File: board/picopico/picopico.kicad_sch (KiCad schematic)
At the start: 52 parts, among them J2 display, J3 USB_B_Micro, Q1 BC817, Q2 BC817, SW1 SW_SPDT, SW3 SW_Push, SW5 SW_Push, SW6 SW_Push, SW7 SW_Push, SW8 SW_Push, U1 ESP32-WROVER-E, U2 volume_wheel, U3 AMS1117-3.3, U4 audio, U5 STC4054GR, U6 CH340C

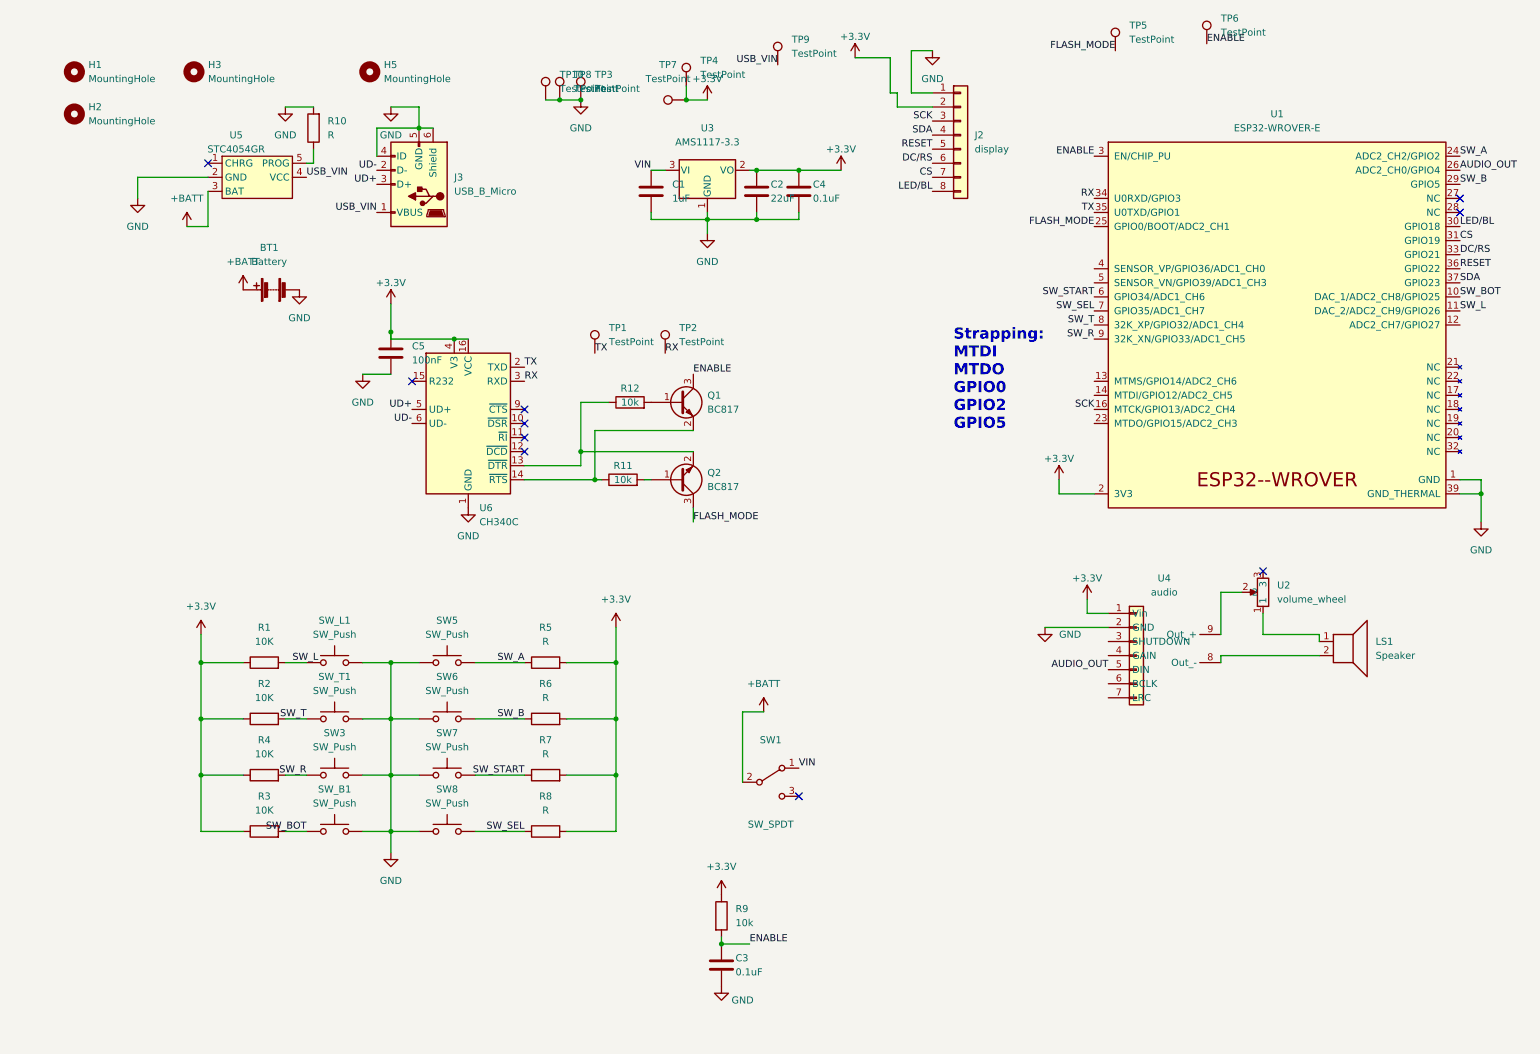
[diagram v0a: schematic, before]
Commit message: more board changes
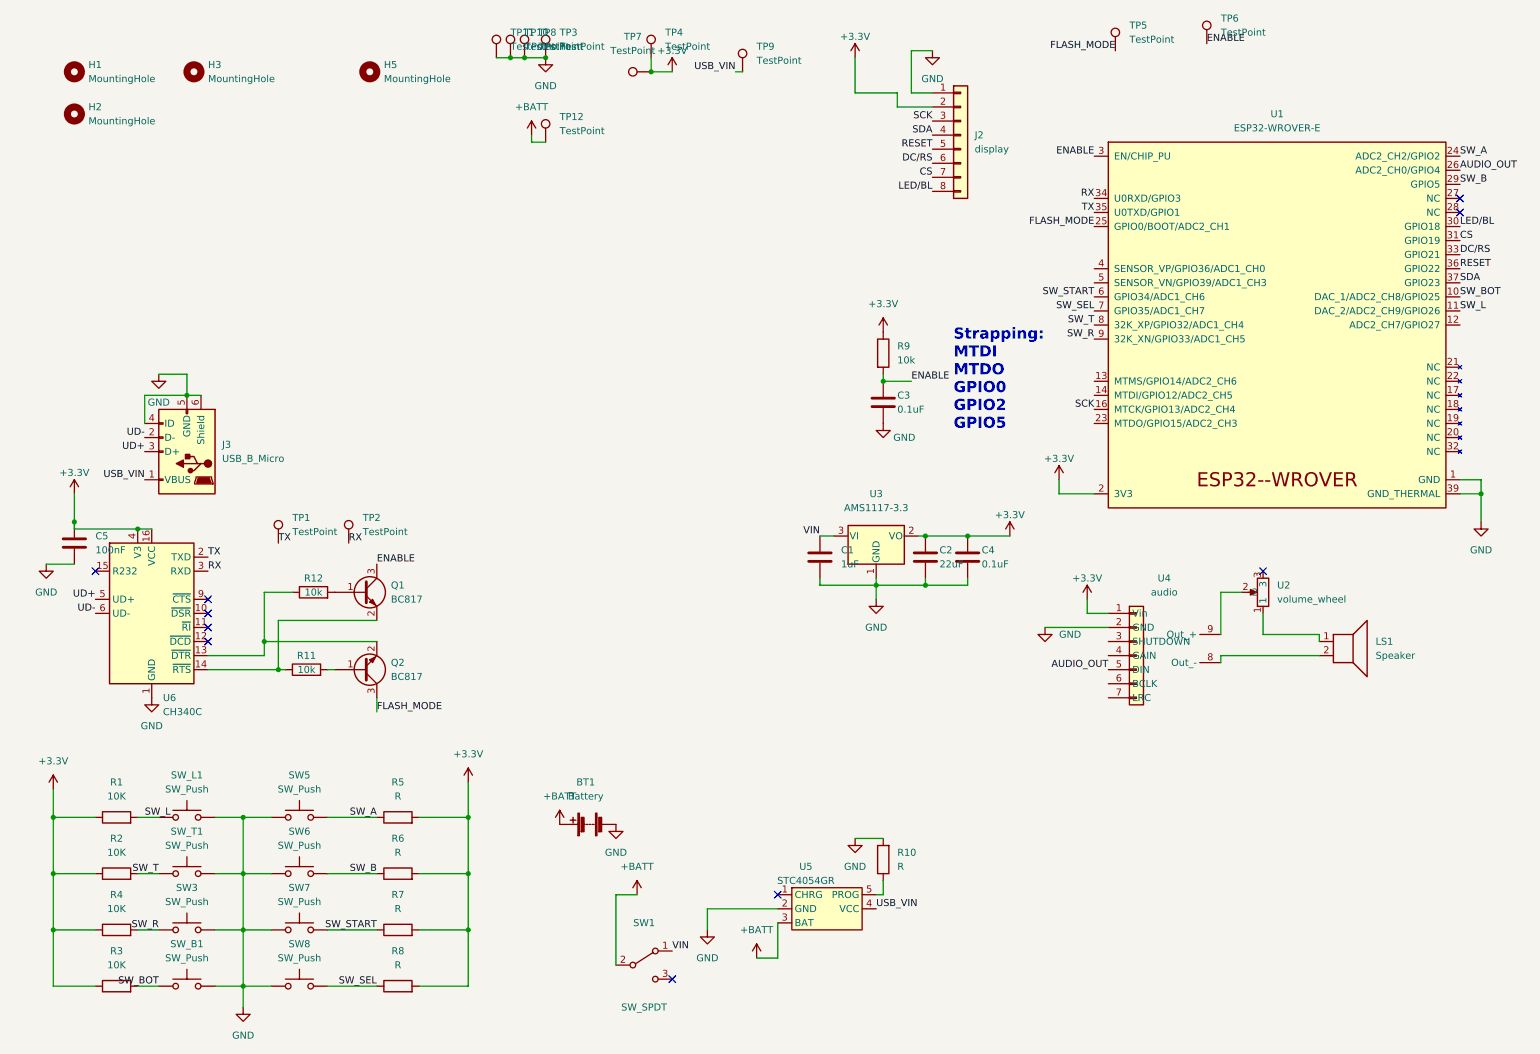
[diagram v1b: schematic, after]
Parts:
- added TP11, TP12: TestPoint, picopico:pad, symbol Connector:TestPoint
- BT1: footprint Connector_JST:JST_PH_S2B-PH-K_1x02_P2.00mm_Horizontal -> picopico:SM02B-SRSS-TB
- SW7, SW8: footprint Button_Switch_SMD:SW_SPST_B3U-1000P -> Button_Switch_SMD:SW_SPST_B3U-1100P-B
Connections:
- net +BATT: now also TP12.1
- net GND: now also TP11.1
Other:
- moved on the sheet: BT1, C1, C2, C3, C4, C5, J3, Q1, Q2, R1, R10, R11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

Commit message: more board stuff
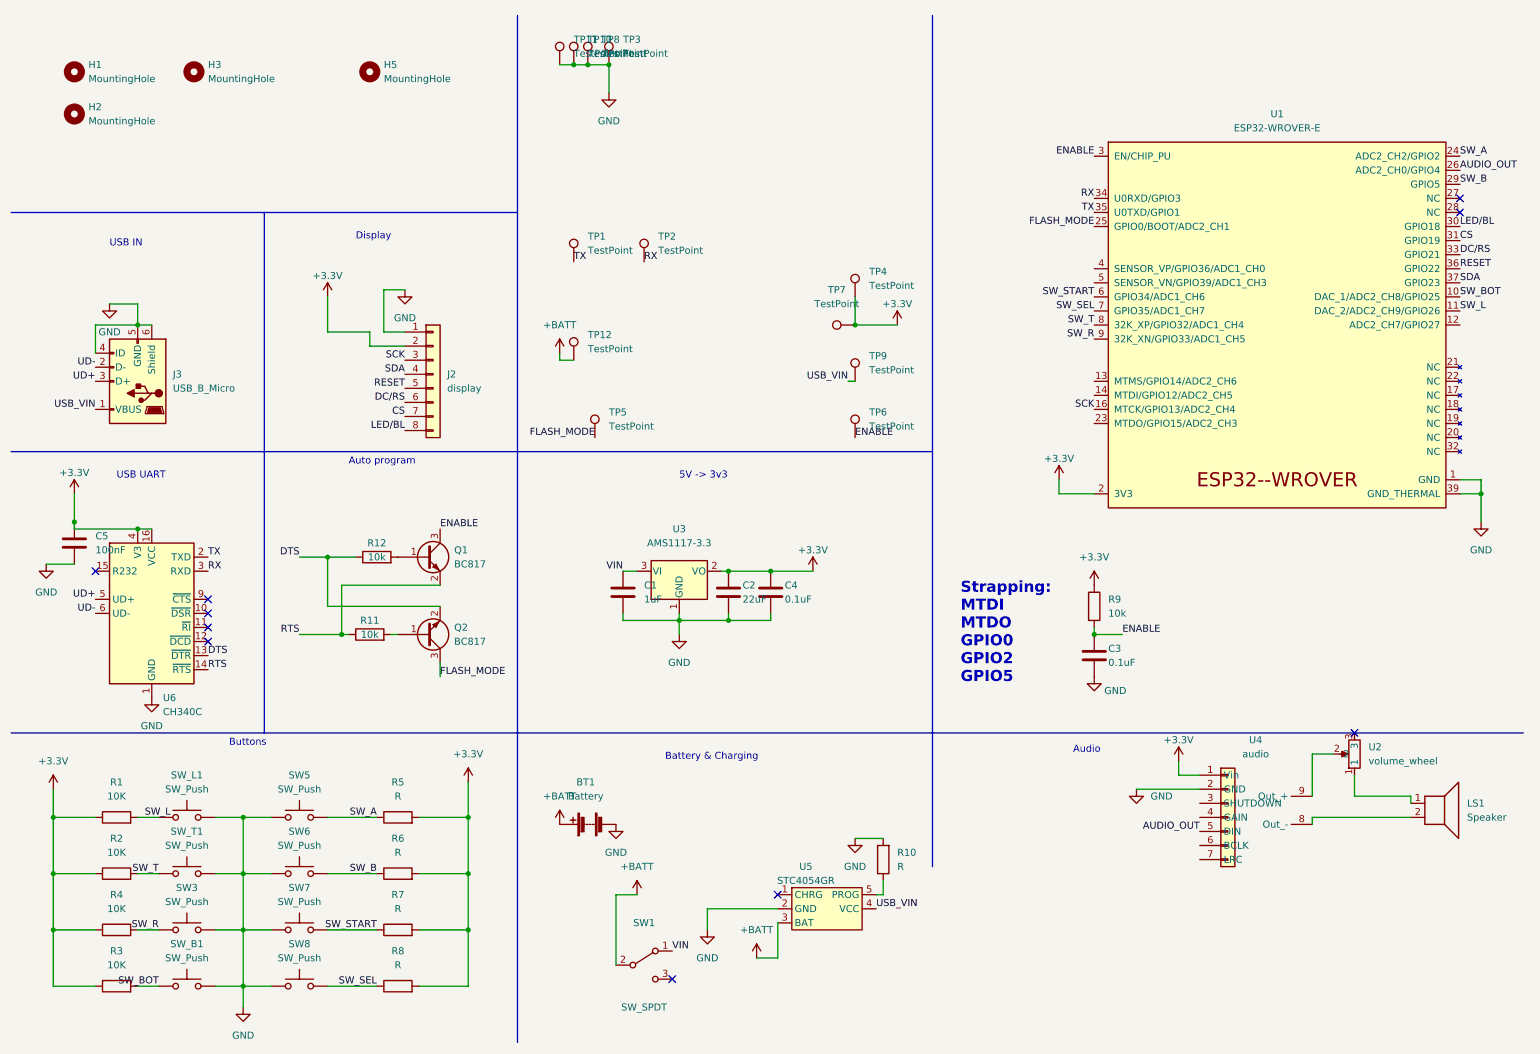
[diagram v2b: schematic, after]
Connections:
- net DTS: now reaches Q2.2 (E), R12.1, U6.13 (~{DTR})
- net RTS: now reaches Q1.2 (E), R11.1, U6.14 (~{RTS})
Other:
- note added: "5V -> 3v3"
- note added: "Audio"
- note added: "Auto program"
- note added: "Battery & Charging"
- note added: "Buttons"
- note added: "Display"
- note added: "USB IN"
- note added: "USB UART"
- moved on the sheet: C1, C2, C3, C4, J2, J3, LS1, Q1, Q2, R11, R12, R9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
